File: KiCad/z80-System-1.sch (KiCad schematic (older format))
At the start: 13 parts, among them J1 FTDI Header, SW1 Reset button, SW2 NMI Button, U1 62256, U2 Z80CPU, U3 AT28C64, U4 16550, U5 74AHC04, X1 ACO-1.8432MHz

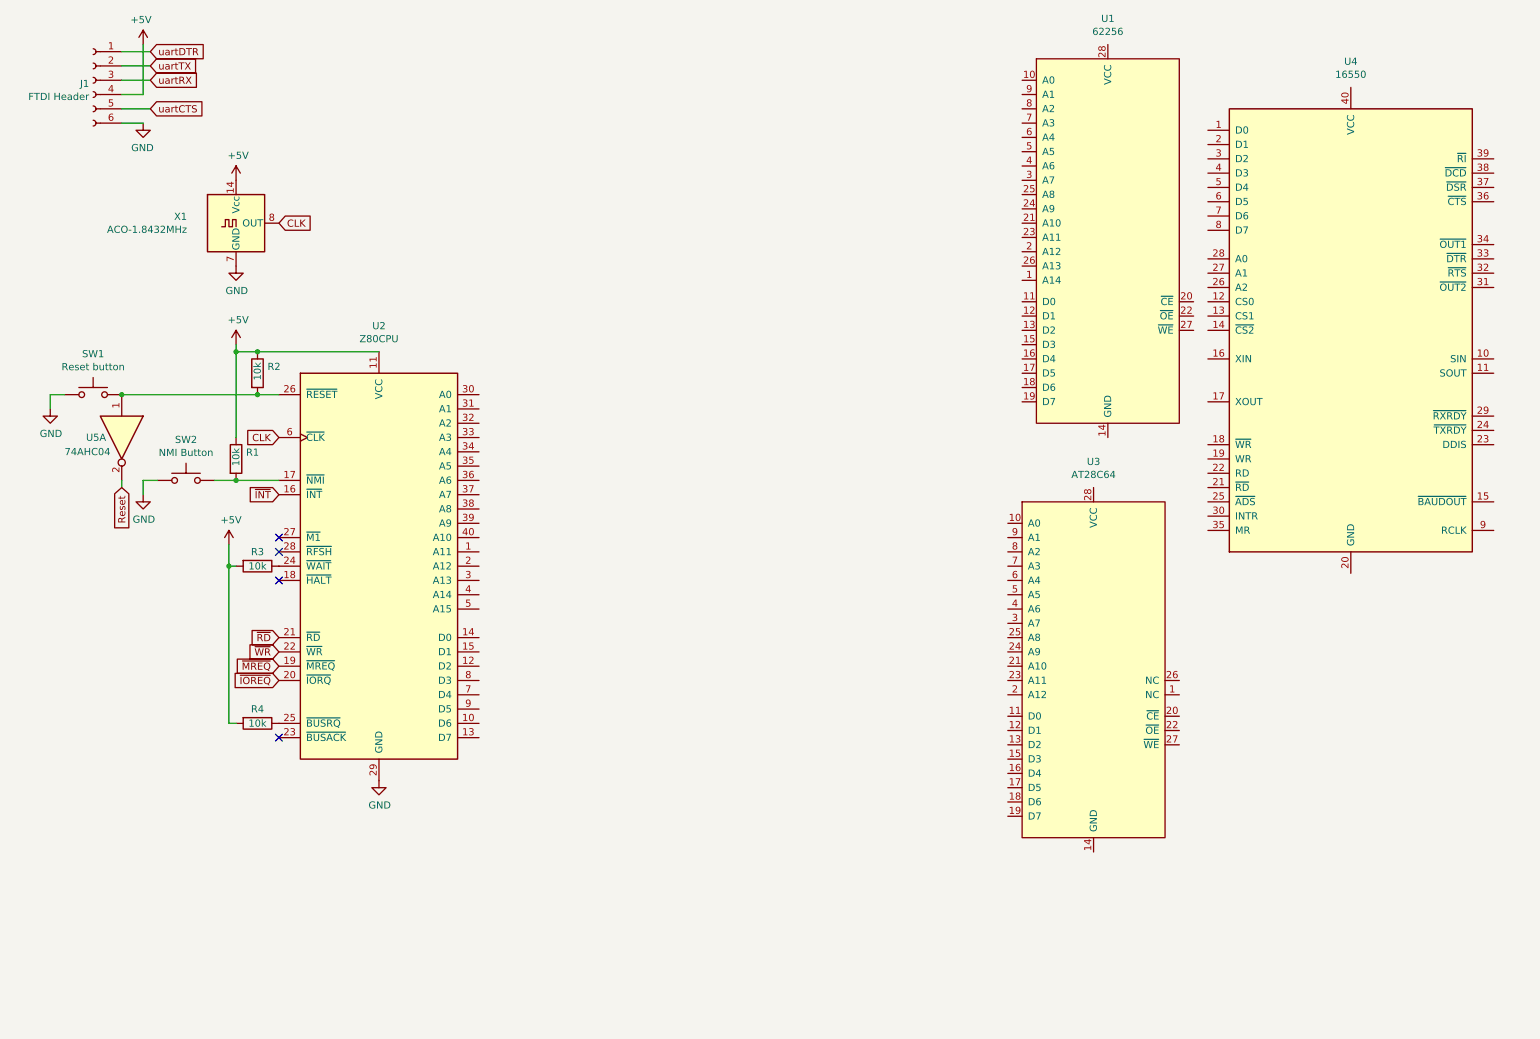
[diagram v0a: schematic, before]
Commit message: Finished schematic and created simple board layout
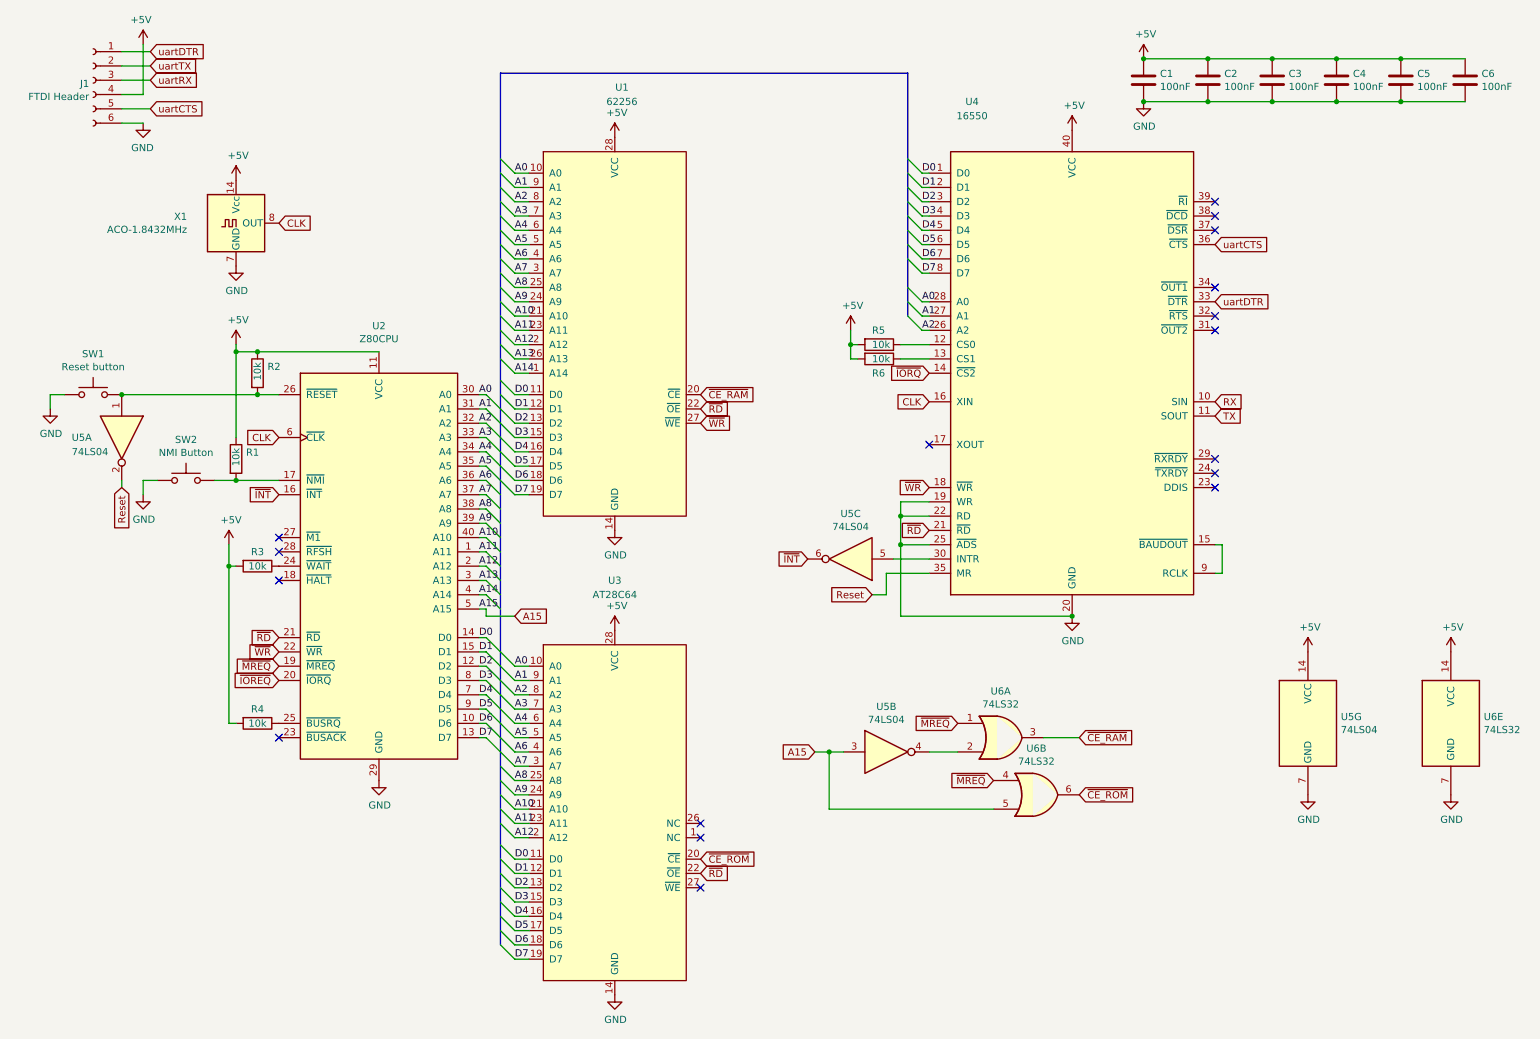
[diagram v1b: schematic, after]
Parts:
- removed U5: 74AHC04, symbol 74xx:74AHC04
- added C1, C2, C3, C4, C5, C6: 100nF, Capacitor_THT:C_Disc_D7.0mm_W2.5mm_P5.00mm, symbol Device:C
- added R5, R6: 10k, Resistor_THT:R_Axial_DIN0204_L3.6mm_D1.6mm_P5.08mm_Horizontal, symbol Device:R
- added U5: 74LS04, symbol 74xx:74LS04
- added U6: 74LS32, symbol 74xx:74LS32
- J1: footprint (none) -> Connector_PinSocket_2.54mm:PinSocket_1x06_P2.54mm_Vertical
- R1, R2, R3, R4: footprint (none) -> Resistor_THT:R_Axial_DIN0204_L3.6mm_D1.6mm_P5.08mm_Horizontal
- SW1, SW2: footprint (none) -> Button_Switch_THT:SW_PUSH_6mm
- U1, U3: footprint (none) -> Package_DIP:DIP-28_W15.24mm
- U2: footprint (none) -> Package_DIP:DIP-40_W15.24mm
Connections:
- net +5V: now also U1.28 (VCC), U3.28 (VCC), U4.40 (VCC), C1.1, C2.1, C3.1, C4.1, C5.1, C6.1, R5.2, R6.2, U5.14 (VCC), U6.14 (VCC)
- net CLK: now also U4.16 (XIN)
- net GND: now also U1.14 (GND), U3.14 (GND), U4.19 (WR), U4.20 (GND), U4.22 (RD), U4.25 (~ADS~), C1.2, C2.2, C3.2, C4.2, C5.2, C6.2, U5.7 (GND), U6.7 (GND)
- net Reset: now also U4.35 (MR), U5.2
- net uartCTS: now also U4.36 (~CTS~)
- net uartDTR: now also U4.33 (~DTR~)
- net ~INT: now also U5.6
- net ~MREQ: now also U6.1, U6.4
- net ~RD: now also U1.22 (~OE), U3.22 (~OE), U4.21 (~RD~)
- net ~WR: now also U1.27 (~WE), U4.18 (~WR~)
- net A14: now reaches U1.1 (A14)
- net A14: now also U2.4 (A14)
- net A0: now reaches U1.10 (A0)
- net A0: now also U2.30 (A0), U3.10 (A0), U4.28 (A0)
- net D0: now reaches U1.11 (D0)
- net D0: now also U2.14 (D0), U3.11 (D0), U4.1 (D0)
- net D1: now reaches U1.12 (D1)
- net D1: now also U2.15 (D1), U3.12 (D1), U4.2 (D1)
- net D2: now reaches U1.13 (D2)
- net D2: now also U2.12 (D2), U3.13 (D2), U4.3 (D2)
- net D3: now reaches U1.15 (D3)
- net D3: now also U2.8 (D3), U3.15 (D3), U4.4 (D3)
- net D4: now reaches U1.16 (D4)
- net D4: now also U2.7 (D4), U3.16 (D4), U4.5 (D4)
- net D5: now reaches U1.17 (D5)
- net D5: now also U2.9 (D5), U3.17 (D5), U4.6 (D5)
- net D6: now reaches U1.18 (D6)
- net D6: now also U2.10 (D6), U3.18 (D6), U4.7 (D6)
- net D7: now reaches U1.19 (D7)
- net D7: now also U2.13 (D7), U3.19 (D7), U4.8 (D7)
- net A12: now reaches U1.2 (A12)
- net A12: now also U2.2 (A12), U3.2 (A12)
- net ~CE_RAM: now reaches U1.20 (~CE)
- net ~CE_RAM: now also U6.3
- net A10: now reaches U1.21 (A10)
- net A10: now also U2.40 (A10), U3.21 (A10)
- net A11: now reaches U1.23 (A11)
- net A11: now also U2.1 (A11), U3.23 (A11)
- net A9: now reaches U1.24 (A9)
- net A9: now also U2.39 (A9), U3.24 (A9)
- net A8: now reaches U1.25 (A8)
- net A8: now also U2.38 (A8), U3.25 (A8)
- net A13: now reaches U1.26 (A13)
- net A13: now also U2.3 (A13)
- net A7: now reaches U1.3 (A7)
- net A7: now also U2.37 (A7), U3.3 (A7)
- net A6: now reaches U1.4 (A6)
- net A6: now also U2.36 (A6), U3.4 (A6)
- net A5: now reaches U1.5 (A5)
- net A5: now also U2.35 (A5), U3.5 (A5)
- net A4: now reaches U1.6 (A4)
- net A4: now also U2.34 (A4), U3.6 (A4)
- net A3: now reaches U1.7 (A3)
- net A3: now also U2.33 (A3), U3.7 (A3)
- net A2: now reaches U1.8 (A2)
- net A2: now also U2.32 (A2), U3.8 (A2), U4.26 (A2)
- net A1: now reaches U1.9 (A1)
- net A1: now also U2.31 (A1), U3.9 (A1), U4.27 (A1)
- net ~CE_ROM: now reaches U3.20 (~CE)
- net ~CE_ROM: now also U6.6
- net at R2.2, SW1.2, U2.26 (~RESET~): now also U5.1
- net A15: now reaches U2.5 (A15)
- net A15: now also U5.3, U6.5
- net RX: now reaches U4.10 (SIN)
- net TX: now reaches U4.11 (SOUT)
- net at U4.12 (CS0): now also R5.1
- net at U4.13 (CS1): now also R6.1
- net ~IORQ: now reaches U4.14 (~CS2~)
- net at U4.15 (~BAUDOUT~): now also U4.9 (RCLK)
- net at U4.30 (INTR): now also U5.5
- new net: U5.4, U6.2
- no-connect marks 4 -> 17
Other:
- moved on the sheet: U1, U3, U4

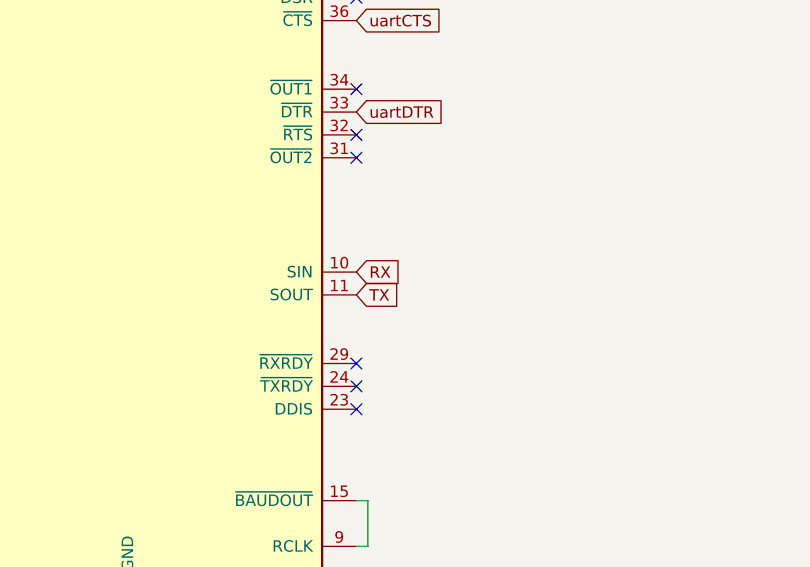
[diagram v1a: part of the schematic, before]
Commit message: Layout 1 finished
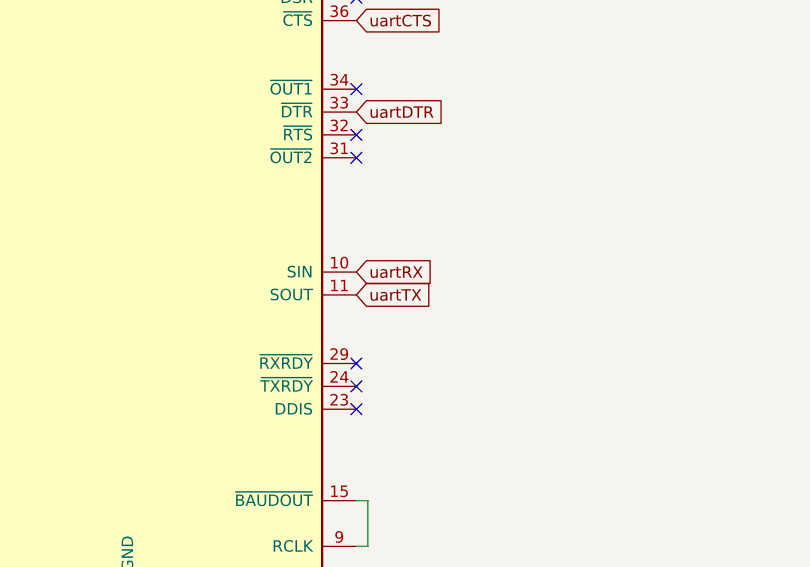
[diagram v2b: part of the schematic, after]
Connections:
- net RX is gone; now on net uartRX: U4.10 (SIN)
- net TX is gone; now on net uartTX: U4.11 (SOUT)
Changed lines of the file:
@@
 NoConn ~ 8850 3650
 Text GLabel 8850 3250 2    50   Input ~ 0
-RX
+uartRX
 Text GLabel 8850 3350 2    50   Input ~ 0
-TX
+uartTX
 Text GLabel 8850 2150 2    50   Input ~ 0
 uartCTS
@@
 Wire Wire Line
 	10150 1150 10600 1150
-Wire Bus Line
-	6700 950  6700 2650
-Wire Bus Line
-	3850 950  3850 7050
 $Comp
 L 74xx:74LS04 U5
@@
 	1    0    0    -1
 $EndComp
+Wire Bus Line
+	6700 950  6700 2650
+Wire Bus Line
+	3850 950  3850 7050
 $EndSCHEMATC
